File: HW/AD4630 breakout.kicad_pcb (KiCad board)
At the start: 2 copper layers, 37.7 x 39.3 mm, 26 parts, among them J1 IN0, J2 IN1, J3 Conn_02x09_Counter_Clockwise, U1 AD4630-24BBCZ, U2 AMS1117-1.8, U3 TXS0108EPW, U4 TXS0108EPW, U6 LTC6655

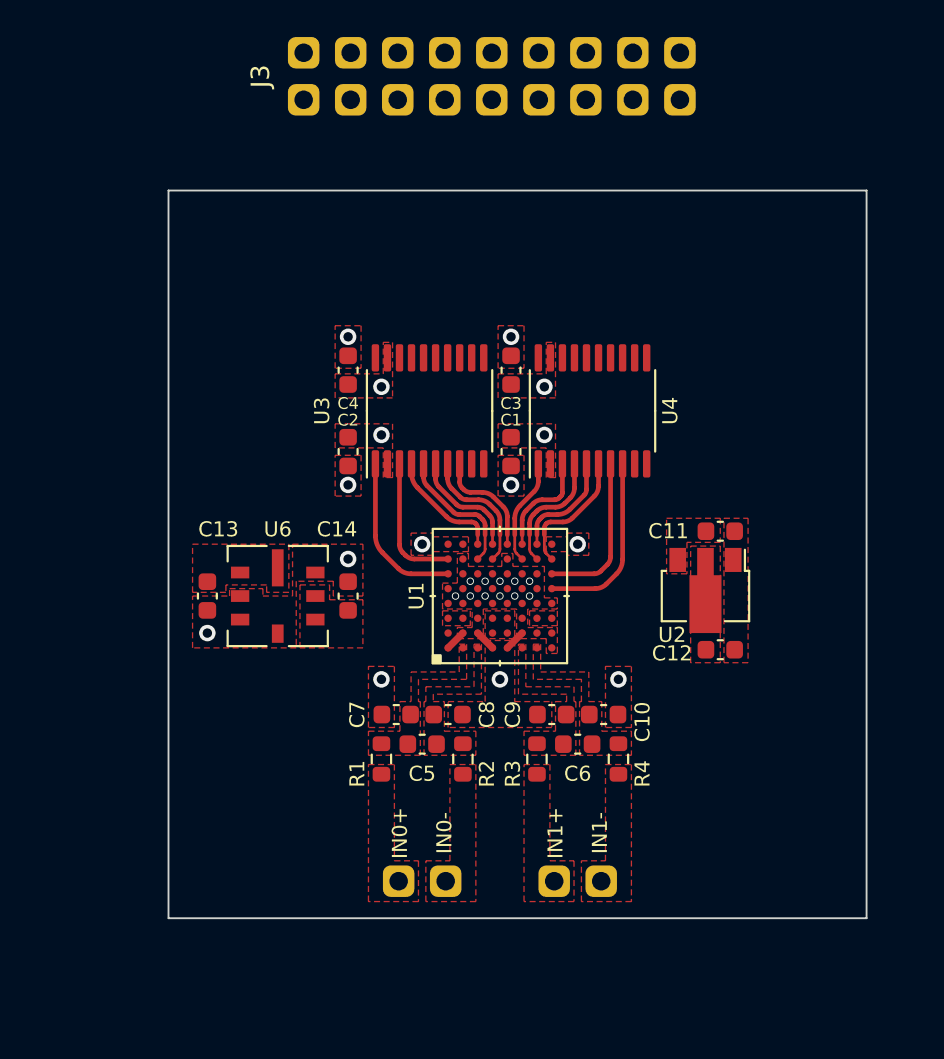
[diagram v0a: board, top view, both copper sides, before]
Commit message: Finished PCB
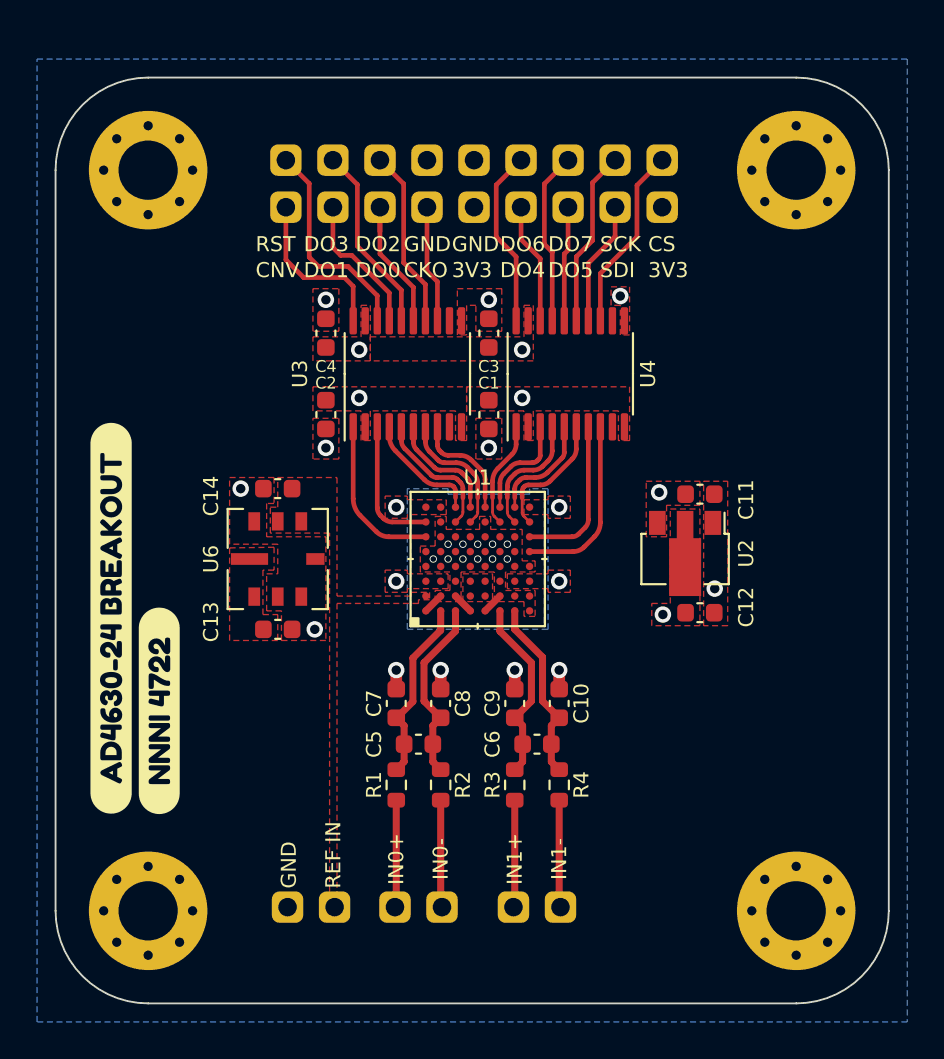
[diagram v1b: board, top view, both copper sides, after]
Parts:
- added H1: MountingHole, MountingHole:MountingHole_3.2mm_M3_Pad_Via, F.Cu at (160.0, 115.0)
- added H2: MountingHole, MountingHole:MountingHole_3.2mm_M3_Pad_Via, F.Cu at (125.0, 115.0)
- added H3: MountingHole, MountingHole:MountingHole_3.2mm_M3_Pad_Via, F.Cu at (125.0, 75.0)
- added H4: MountingHole, MountingHole:MountingHole_3.2mm_M3_Pad_Via, F.Cu at (160.0, 75.0)
- added J4: IN0, Connector_PinHeader_2.54mm:PinHeader_1x02_P2.54mm_Vertical, F.Cu at (135.1, 114.8)
- added kibuzzard-638251C8: G***, kibuzzard-638251C8, F.Cu at (123.0, 99.2)
- added kibuzzard-638251EC: G***, kibuzzard-638251EC, F.Cu at (125.6, 104.2)
- moved C14 6.93 mm to (132.0, 92.2), turned to 180 degrees
- moved J3 5.88 mm to (132.4, 77.0)
- moved C13 4.20 mm to (132.0, 99.8), turned to 0 degrees
- moved R4 3.49 mm to (147.2, 108.2)
- moved J2 2.61 mm to (144.7, 114.8)
- moved C10 2.47 mm to (147.2, 103.8), turned to -90 degrees
- moved C2 2.33 mm to (134.6, 88.2)
- moved C4 2.33 mm to (134.6, 83.8)
- moved U4 2.33 mm to (147.8, 86.0)
- moved C1 2.33 mm to (143.4, 88.2)
- moved C3 2.33 mm to (143.4, 83.8)
- moved U1 2.33 mm to (142.8, 96.0)
- moved U3 2.33 mm to (139.0, 86.0)
- moved C11 2.28 mm to (154.8, 92.5)
- moved C12 2.28 mm to (154.8, 98.9)
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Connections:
- C11 pad 1: +5V -> +3V3
- C3 pad 1: +5V -> +3V3
- C4 pad 1: +5V -> +3V3
- J3 pad 1: /OE -> /CNV/
- J3 pad 10: /OE1 -> GND
- J3 pad 11: Net-(U4-Pad20) -> /SDO4/
- J3 pad 12: Net-(U4-Pad18) -> /SDO6/
- J3 pad 13: Net-(U4-Pad17) -> /SDO5/
- J3 pad 14: Net-(U4-Pad16) -> /SDO7/
- J3 pad 15: Net-(U4-Pad15) -> /SDI/
- J3 pad 16: Net-(U4-Pad14) -> /SCK/
- J3 pad 17: Net-(U4-Pad13) -> +3V3
- J3 pad 18: Net-(U4-Pad12) -> /CS/
- J3 pad 2: Net-(U3-Pad20) -> /RST/
- J3 pad 3: Net-(U3-Pad18) -> /SDO1/
- J3 pad 4: Net-(U3-Pad17) -> /SDO3/
- J3 pad 5: Net-(U3-Pad16) -> /SDO0/
- J3 pad 6: Net-(U3-Pad15) -> /SDO2/
- J3 pad 7: Net-(U3-Pad14) -> /SCKo/
- J3 pad 8: Net-(U3-Pad13) -> GND
- J3 pad 9: Net-(U3-Pad12) -> +3V3
- U2 pad 3: +5V -> +3V3
- U3 pad 10: /OE -> +1V8
- U3 pad 12: Net-(U3-Pad12) -> unconnected-(U3-Pad12)
- U3 pad 13: Net-(U3-Pad13) -> /SCKo/
- U3 pad 14: Net-(U3-Pad14) -> /SDO2/
- U3 pad 15: Net-(U3-Pad15) -> /SDO0/
- U3 pad 16: Net-(U3-Pad16) -> /SDO3/
- U3 pad 17: Net-(U3-Pad17) -> /SDO1/
- U3 pad 18: Net-(U3-Pad18) -> /RST/
- U3 pad 19: +5V -> +3V3
- U3 pad 20: Net-(U3-Pad20) -> /CNV/
- U4 pad 10: /OE1 -> +1V8
- U4 pad 12: Net-(U4-Pad12) -> unconnected-(U4-Pad12)
- U4 pad 13: Net-(U4-Pad13) -> /CS/
- U4 pad 14: Net-(U4-Pad14) -> /SDI/
- U4 pad 15: Net-(U4-Pad15) -> /SCK/
- U4 pad 16: Net-(U4-Pad16) -> /SDO5/
- U4 pad 17: Net-(U4-Pad17) -> /SDO7/
- U4 pad 18: Net-(U4-Pad18) -> /SDO4/
- U4 pad 19: +5V -> +3V3
- U4 pad 20: Net-(U4-Pad20) -> /SDO6/
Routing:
- net /RST/: track 0.00 -> 11.7 mm
- net /SDO3/: track 0.00 -> 10.2 mm
- net /CS/: track 0.00 -> 10.1 mm
- net /IN1+: track 0.00 -> 10.0 mm
- net /IN0-: track 0.00 -> 10.0 mm
- net /IN0+: track 0.00 -> 9.94 mm
- net /IN1-: track 0.00 -> 9.92 mm
- net /SDO2/: track 0.00 -> 9.69 mm
- net /SDO6/: track 0.00 -> 9.68 mm
- net /SCK/: track 0.00 -> 9.55 mm
- net /SDO7/: track 0.00 -> 9.38 mm
- net /CNV/: track 0.00 -> 8.93 mm
- net /SDO1/: track 0.00 -> 7.75 mm
- net /SDO0/: track 0.00 -> 7.54 mm
- net /SDI/: track 0.00 -> 6.74 mm
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- added copper zone on In2.Cu, net +1V8
- added copper zone on F.Cu, net +3V3
- added copper zone on In2.Cu, net +3V3
- added copper zone on B.Cu, net GND
- added copper zone on In1.Cu, net GND
- added copper zone on In2.Cu, net GND
- removed copper zone on F.Cu, net /IN0+
- removed copper zone on F.Cu, net /IN0-
- removed copper zone on F.Cu, net /IN1+
- removed copper zone on F.Cu, net /IN1-
- removed copper zone on F.Cu, net Net-(J1-Pad1)
- removed copper zone on F.Cu, net Net-(J1-Pad2)
- removed copper zone on F.Cu, net Net-(J2-Pad1)
- removed copper zone on F.Cu, net Net-(J2-Pad2)
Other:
- board size 37.7 x 39.3 mm -> 45 x 50 mm
- copper layers 2 -> 4
- board text added: "3V3"
- board text added: "CKO"
- board text added: "CNV"
- board text added: "CS"
- board text added: "DO0"
- board text added: "DO1"
- board text added: "DO2"
- board text added: "DO3"
- board text added: "DO4"
- board text added: "DO5"
- board text added: "DO6"
- board text added: "DO7"
- board text added: "GND"
- board text added: "REF IN"
- board text added: "RST"
- board text added: "SCK"
- board text added: "SDI"
